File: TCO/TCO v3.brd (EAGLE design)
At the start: 60.6 x 82.5 mm, 19 parts

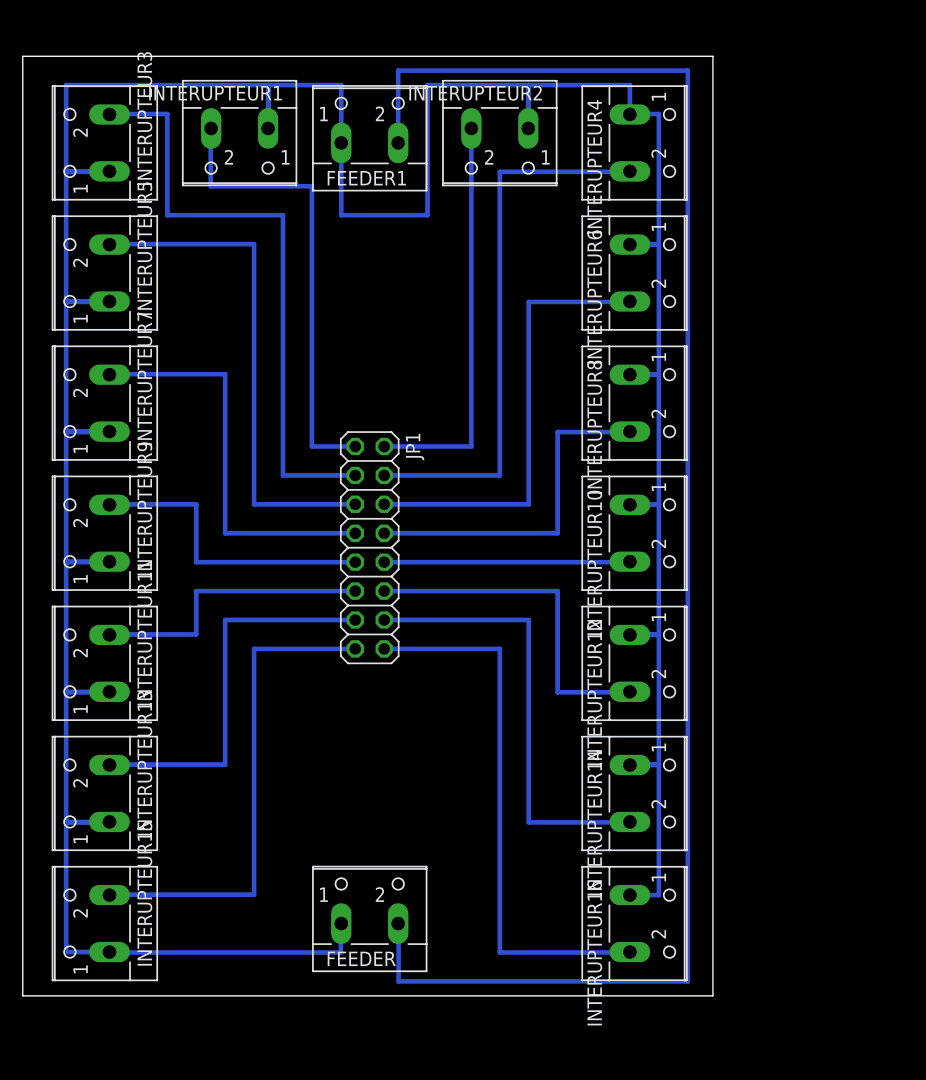
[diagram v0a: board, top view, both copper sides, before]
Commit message: update
optimisation de mmontage
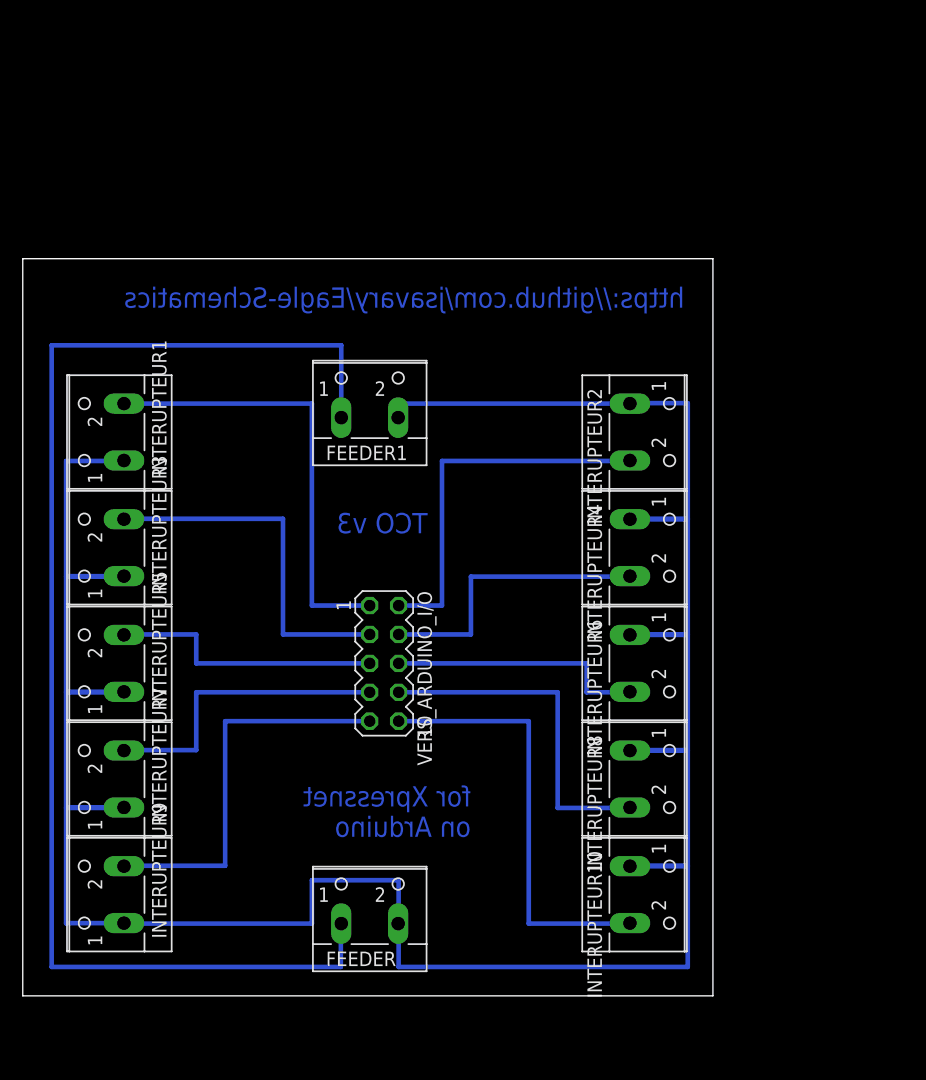
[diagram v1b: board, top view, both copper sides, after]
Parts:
- removed INTERUPTEUR11, INTERUPTEUR12, INTERUPTEUR13, INTERUPTEUR14, INTERUPTEUR15, INTERUPTEUR16: (no value), con-wago-500:W237-102
- removed JP1: (no value), pinhead:2X08
- added VERS_ARDUINO_I/O: (no value), con-lstb:MA05-2
- moved INTERUPTEUR3 35.6 mm to (47.0, 43.2)
- moved INTERUPTEUR4 35.6 mm to (94.0, 43.2)
- moved INTERUPTEUR5 34.3 mm to (47.0, 33.0)
- moved INTERUPTEUR6 34.3 mm to (94.0, 33.0)
- moved INTERUPTEUR7 33.0 mm to (47.0, 22.9)
- moved INTERUPTEUR8 33.0 mm to (94.0, 22.9)
- moved INTERUPTEUR9 31.8 mm to (47.0, 12.7)
- moved INTERUPTEUR10 31.8 mm to (94.0, 12.7)
- moved INTERUPTEUR2 28.4 mm to (94.0, 53.3), turned to 270 degrees
- moved INTERUPTEUR1 27.9 mm to (47.0, 53.3), turned to 90 degrees
- moved FEEDER1 24.1 mm to (69.8, 55.9)
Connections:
- removed net N$12: INTERUPTEUR10.2, JP1.10
- removed net N$13: INTERUPTEUR11.2, JP1.11
- removed net N$14: INTERUPTEUR12.2, JP1.12
- removed net N$15: INTERUPTEUR13.2, JP1.13
- removed net N$16: INTERUPTEUR14.2, JP1.14
- removed net N$17: INTERUPTEUR15.2, JP1.15
- removed net N$18: INTERUPTEUR16.2, JP1.16
- new net N$26: FEEDER.2, FEEDER1.2, INTERUPTEUR1.1, INTERUPTEUR10.1, INTERUPTEUR2.1, INTERUPTEUR3.1, INTERUPTEUR4.1, INTERUPTEUR5.1, INTERUPTEUR6.1, INTERUPTEUR7.1, INTERUPTEUR8.1, INTERUPTEUR9.1
- net N$1: no longer INTERUPTEUR1.1, INTERUPTEUR10.1, INTERUPTEUR11.1, INTERUPTEUR12.1, INTERUPTEUR13.1, INTERUPTEUR14.1, INTERUPTEUR15.1, INTERUPTEUR16.1, INTERUPTEUR2.1, INTERUPTEUR3.1, INTERUPTEUR4.1, INTERUPTEUR5.1, INTERUPTEUR6.1, INTERUPTEUR7.1, INTERUPTEUR8.1, INTERUPTEUR9.1
- net N$10: now also VERS_ARDUINO_I/O.8; no longer JP1.8
- net N$11: now also INTERUPTEUR10.2, VERS_ARDUINO_I/O.10; no longer INTERUPTEUR9.2, JP1.9
- net N$2: now also INTERUPTEUR1.2, VERS_ARDUINO_I/O.1; no longer FEEDER.2, FEEDER1.2
- net N$3: now also INTERUPTEUR3.2, VERS_ARDUINO_I/O.3; no longer INTERUPTEUR1.2, JP1.1
- net N$4: now also INTERUPTEUR5.2, VERS_ARDUINO_I/O.5; no longer INTERUPTEUR2.2, JP1.2
- net N$5: now also INTERUPTEUR7.2, VERS_ARDUINO_I/O.7; no longer INTERUPTEUR3.2, JP1.3
- net N$6: now also INTERUPTEUR9.2, VERS_ARDUINO_I/O.9; no longer INTERUPTEUR4.2, JP1.4
- net N$7: now also INTERUPTEUR2.2, VERS_ARDUINO_I/O.2; no longer INTERUPTEUR5.2, JP1.5
- net N$8: now also INTERUPTEUR4.2, VERS_ARDUINO_I/O.4; no longer INTERUPTEUR6.2, JP1.6
- net N$9: now also INTERUPTEUR6.2, VERS_ARDUINO_I/O.6; no longer INTERUPTEUR7.2, JP1.7
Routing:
- net N$26: track 0.00 -> 259.6 mm
- net N$1: track 338.5 -> 115.7 mm
- net N$2: track 142.3 -> 39.3 mm
- net N$18: track 48.3 -> 0.00 mm
- net N$17: track 43.2 -> 0.00 mm
- net N$16: track 39.4 -> 0.00 mm
- net N$15: track 34.3 -> 0.00 mm
- net N$14: track 30.5 -> 0.00 mm
- net N$5: track 53.4 -> 26.7 mm
- net N$13: track 25.4 -> 0.00 mm
- net N$12: track 21.6 -> 0.00 mm
- net N$8: track 39.4 -> 25.4 mm
- net N$6: track 48.3 -> 34.3 mm
- net N$9: track 35.6 -> 22.9 mm
- net N$4: track 35.6 -> 24.2 mm
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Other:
- board size 60.6 x 82.5 mm -> 60.6 x 64.8 mm
- board text added: "TCO v3"
- board text added: "for Xpressnet on Arduino"
- board text added: "https://github.com/jsavary/Eagle-Schematics"
